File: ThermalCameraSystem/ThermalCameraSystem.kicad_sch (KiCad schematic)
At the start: 3 parts, among them U1 MLX90621ESF-BAB-000-SP

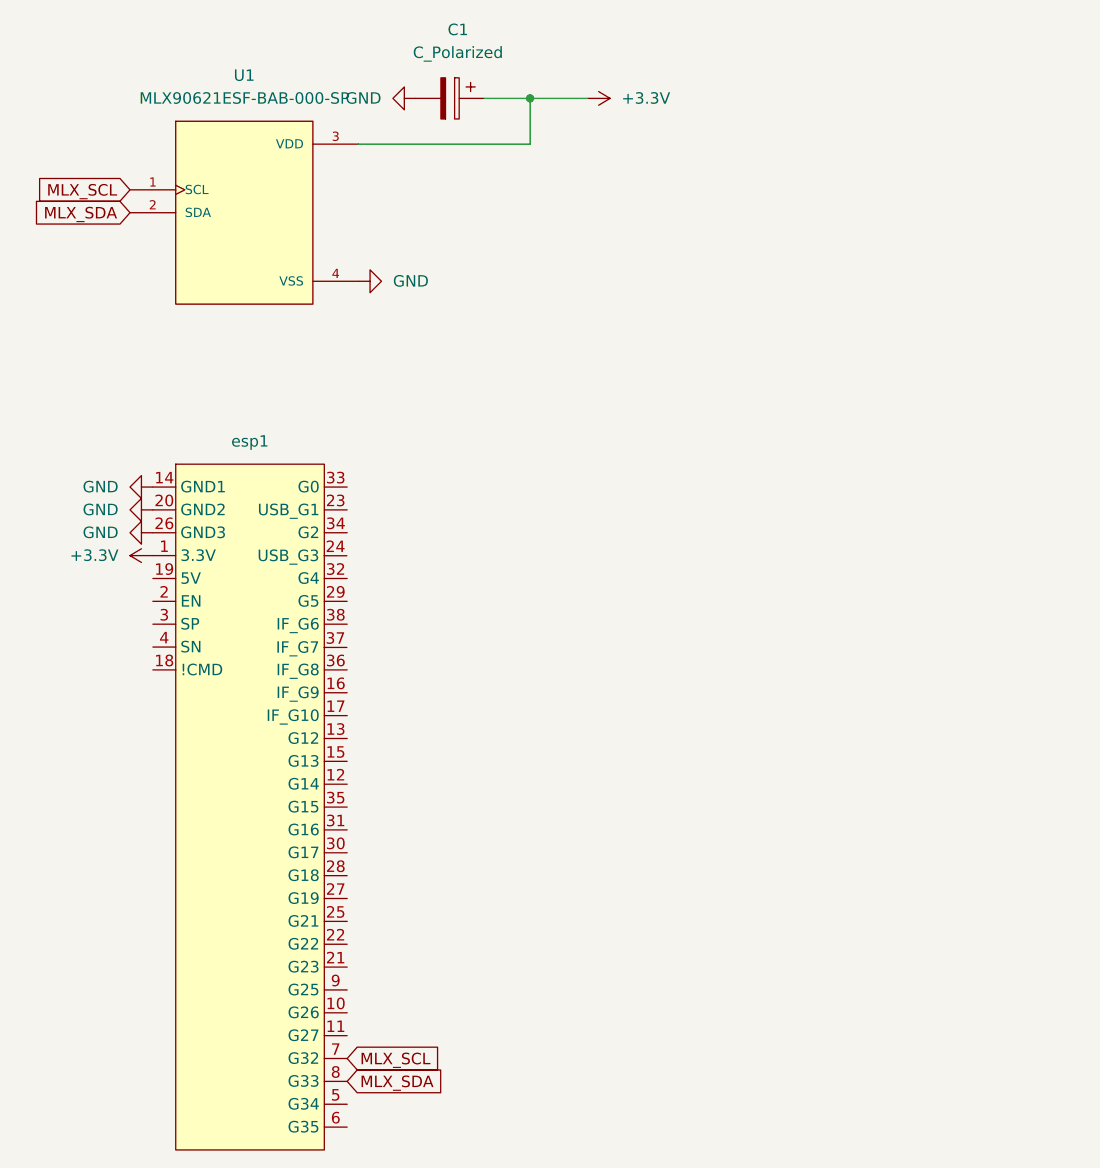
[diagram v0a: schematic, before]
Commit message: Updated main
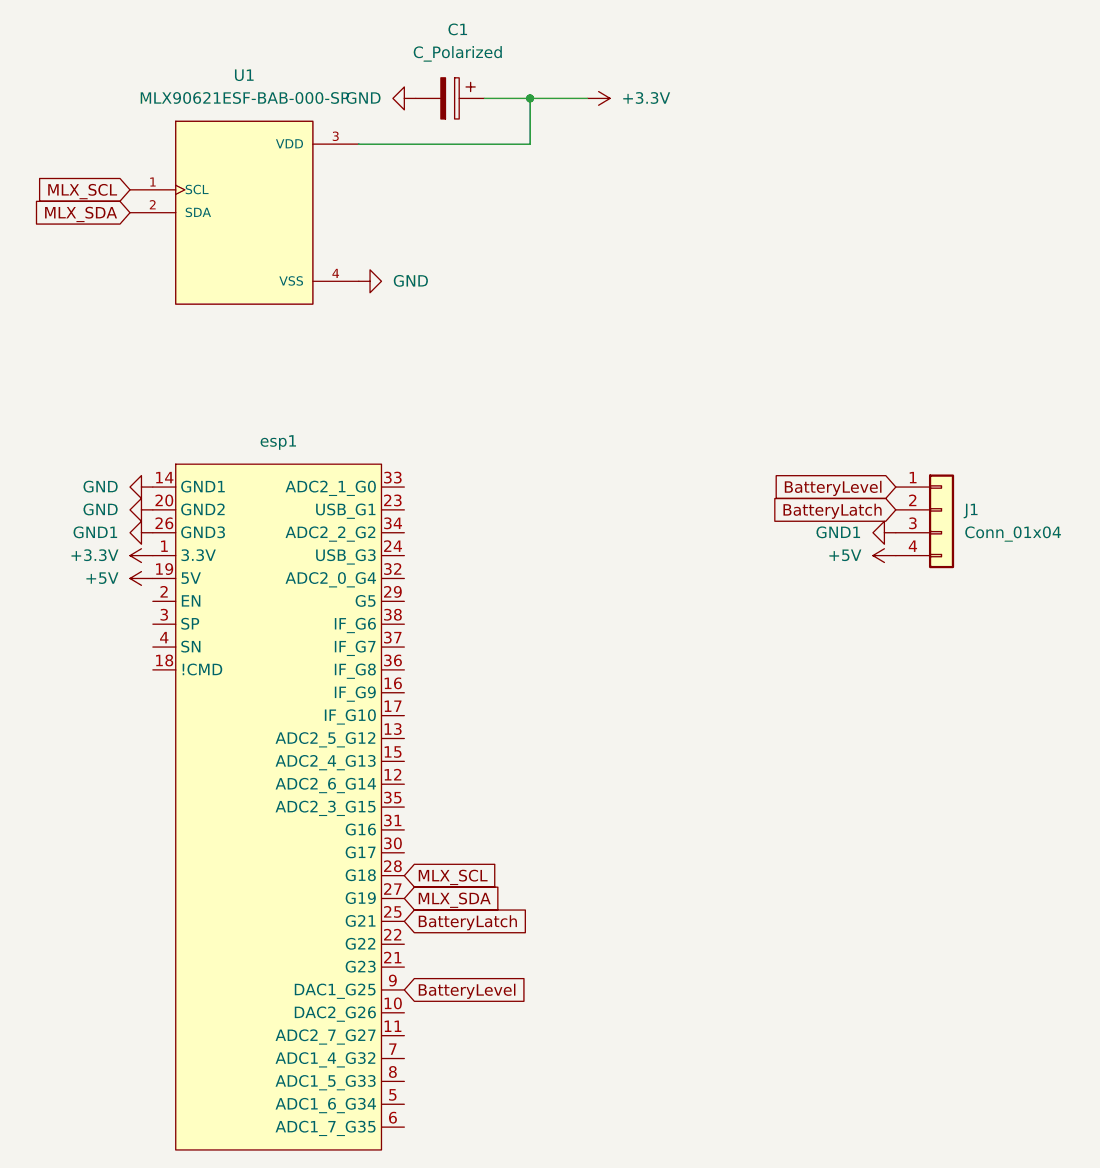
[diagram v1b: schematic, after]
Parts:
- added J1: Conn_01x04, Connector_PinSocket_2.54mm:PinSocket_1x04_P2.54mm_Vertical, symbol Connector_Generic:Conn_01x04
- U1: footprint TO254P940H1340-4:TO254P940H1340-4 -> TO292P930H600-4
- esp1: footprint Library:AZdelivery_nodemcu_esp32 -> AZdelivery_nodemcu_esp32
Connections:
- net GND: no longer esp1.26 (GND3)
- net MLX_SCL: now also esp1.28 (G18); no longer esp1.7 (G32)
- net MLX_SDA: now also esp1.27 (G19); no longer esp1.8 (G33)
- net +5V: now reaches esp1.19 (5V)
- net +5V: now also J1.4 (Pin_4)
- net BatteryLatch: now reaches esp1.25 (G21)
- net BatteryLatch: now also J1.2 (Pin_2)
- net BatteryLevel: now reaches esp1.9 (DAC1_G25)
- net BatteryLevel: now also J1.1 (Pin_1)
- new net GND1: J1.3 (Pin_3), esp1.26 (GND3)
